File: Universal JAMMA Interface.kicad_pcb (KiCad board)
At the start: 2 copper layers, 111 x 60.8 mm, 31 parts, among them U1 LM386, U2 DIP-14_W7.62mm_Socket

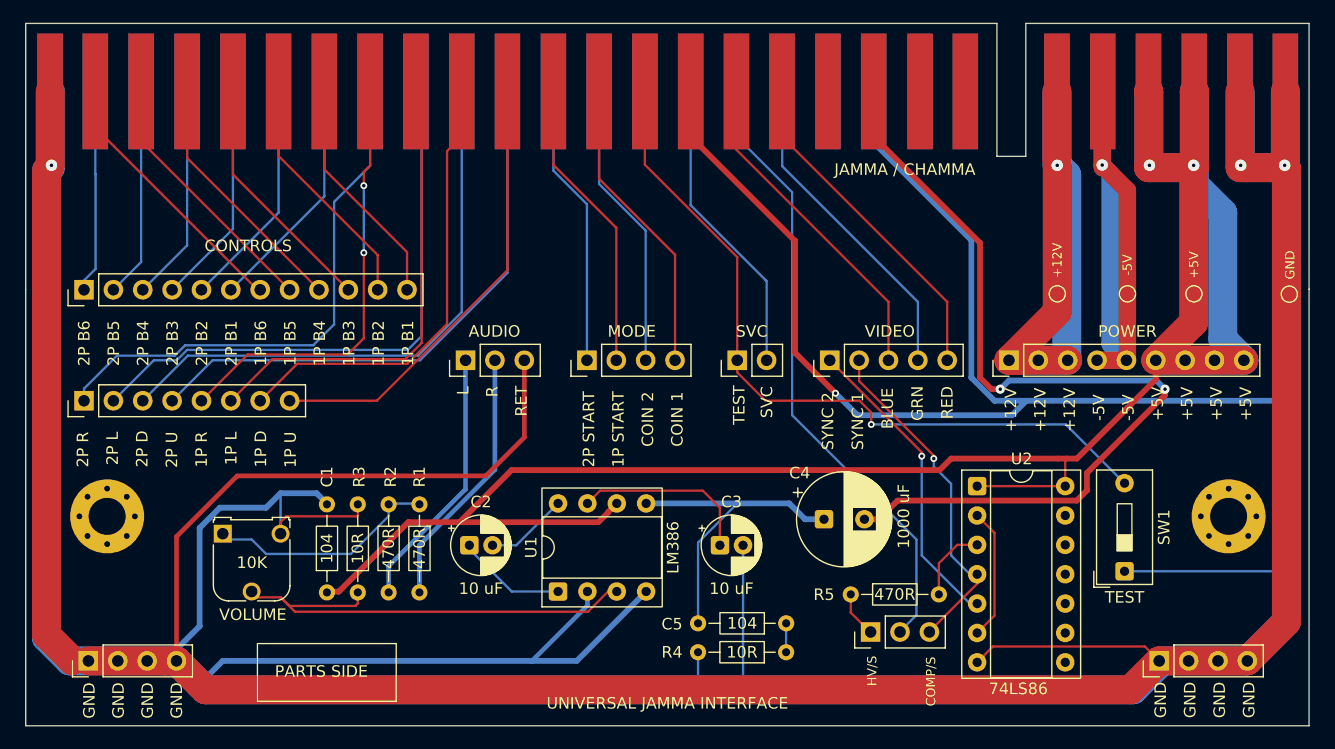
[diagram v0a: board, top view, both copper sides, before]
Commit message: slightly widen
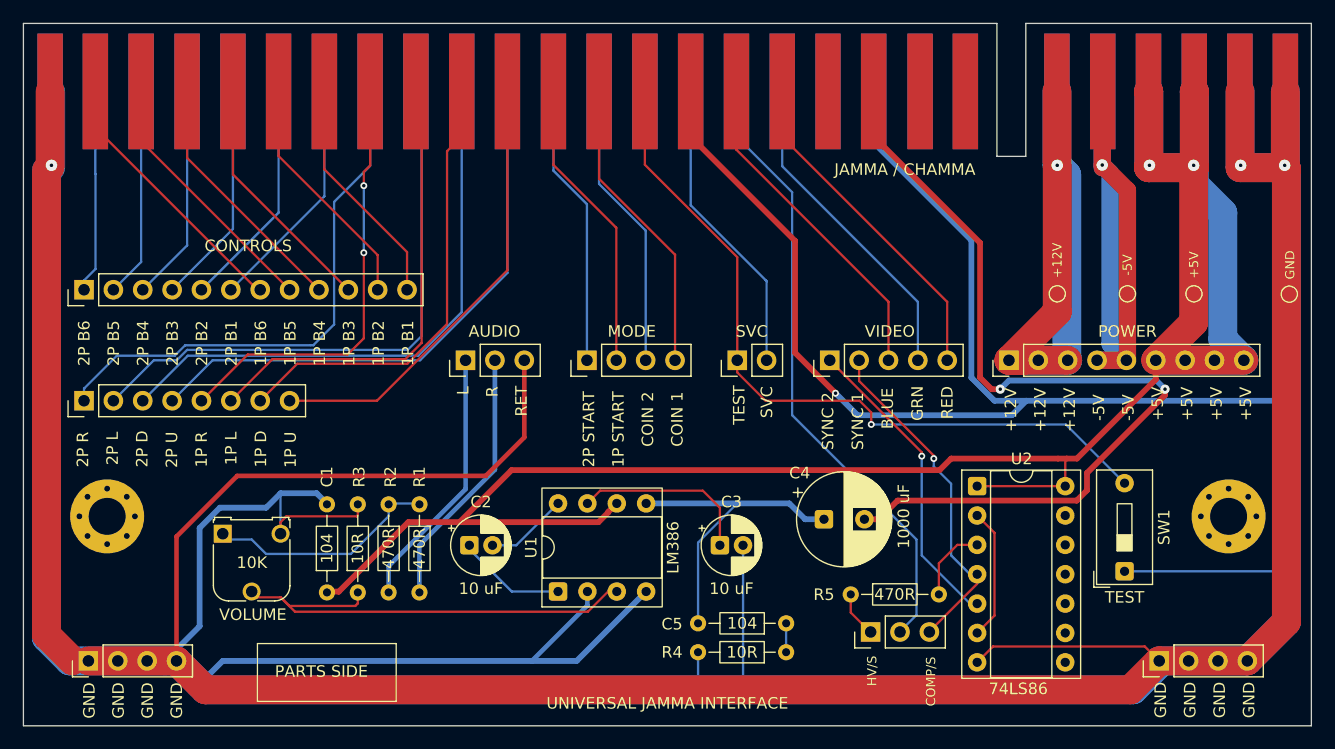
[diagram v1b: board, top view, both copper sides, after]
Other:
- board size 111 x 60.8 mm -> 111.4 x 60.8 mm
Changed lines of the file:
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@@
 	(gr_poly
 		(pts
-			(xy 204.957988 124.1125) (xy 93.957985 124.1125) (xy 93.957985 86.3625) (xy 93.957985 63.362495)
-			(xy 177.957988 63.362495) (xy 177.957988 74.8625) (xy 180.457988 74.8625) (xy 180.457988 63.362495)
-			(xy 204.957992 63.362495) (xy 204.957992 86.3625) (xy 204.957988 86.3625)
+			(xy 205.157988 124.1125) (xy 93.757985 124.1125) (xy 93.757985 63.362495) (xy 177.957988 63.362495)
+			(xy 177.957988 74.8625) (xy 180.457988 74.8625) (xy 180.457988 63.362495) (xy 205.157992 63.362495)
 		)
 		(stroke
